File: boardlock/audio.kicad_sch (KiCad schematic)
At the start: 7 parts, among them U7 MAX98357AETE+T

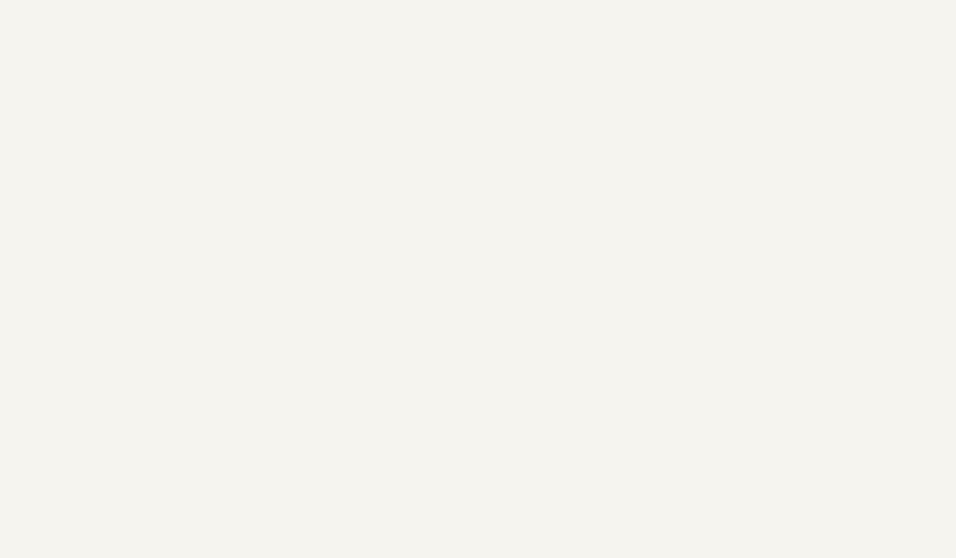
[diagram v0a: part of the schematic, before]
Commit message: modifications?
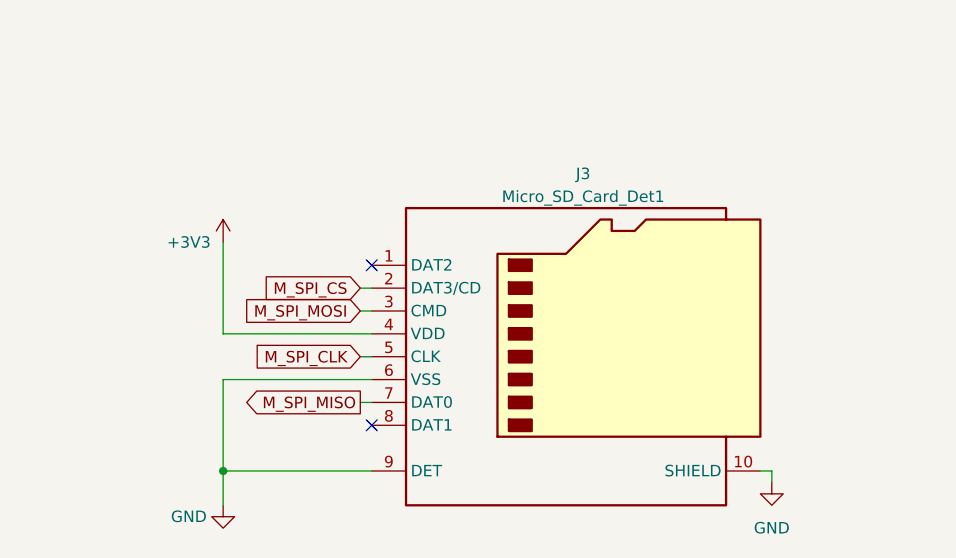
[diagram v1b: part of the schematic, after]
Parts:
- added J3: Micro_SD_Card_Det1, symbol Connector:Micro_SD_Card_Det1
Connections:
- net +3V3: now also J3.4 (VDD)
- net GND: now also J3.10 (SHIELD), J3.6 (VSS), J3.9 (DET)
- new net M_SPI_CLK: J3.5 (CLK)
- new net M_SPI_CS: J3.2 (DAT3/CD)
- new net M_SPI_MISO: J3.7 (DAT0)
- new net M_SPI_MOSI: J3.3 (CMD)
- no-connect marks 0 -> 2
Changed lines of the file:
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@@
   (junction (at 171.45 124.46) (diameter 0) (color 0 0 0 0)
   )
+  (junction (at 73.66 146.05) (diameter 0) (color 0 0 0 0)
+  )
   (junction (at 59.69 53.34) (diameter 0) (color 0 0 0 0)
   )
@@
   (junction (at 219.71 130.81) (diameter 0) (color 0 0 0 0)
   )
+  (no_connect (at 90.17 140.97))
+  (no_connect (at 90.17 123.19))
+  (wire (pts (xy 73.66 149.86) (xy 73.66 146.05))
+    (stroke (width 0) (type default))
+  )
   (wire (pts (xy 219.71 130.81) (xy 219.71 133.35))
     (stroke (width 0) (type default))
   )
+  (wire (pts (xy 134.62 146.05) (xy 134.62 147.32))
+    (stroke (width 0) (type default))
+  )
   (wire (pts (xy 41.91 39.37) (xy 52.07 39.37))
     (stroke (width 0) (type default))
@@
     (stroke (width 0) (type default))
   )
+  (wire (pts (xy 73.66 146.05) (xy 73.66 135.89))
+    (stroke (width 0) (type default))
+  )
   (wire (pts (xy 59.69 76.2) (xy 59.69 81.28))
     (stroke (width 0) (type default))
   )
+  (wire (pts (xy 88.9 125.73) (xy 90.17 125.73))
+    (stroke (width 0) (type default))
+  )
   (wire (pts (xy 59.69 76.2) (xy 62.23 76.2))
     (stroke (width 0) (type default))
@@
     (stroke (width 0) (type default))
   )
+  (wire (pts (xy 90.17 133.35) (xy 88.9 133.35))
+    (stroke (width 0) (type default))
+  )
   (wire (pts (xy 41.91 36.83) (xy 41.91 39.37))
     (stroke (width 0) (type default))
@@
     (stroke (width 0) (type default))
   )
+  (wire (pts (xy 73.66 146.05) (xy 90.17 146.05))
+    (stroke (width 0) (type default))
+  )
   (wire (pts (xy 181.61 121.92) (xy 185.42 121.92))
     (stroke (width 0) (type default))
@@
     (stroke (width 0) (type default))
   )
+  (wire (pts (xy 73.66 135.89) (xy 90.17 135.89))
+    (stroke (width 0) (type default))
+  )
+  (wire (pts (xy 90.17 128.27) (xy 88.9 128.27))
+    (stroke (width 0) (type default))
+  )
   (wire (pts (xy 97.79 77.47) (xy 101.6 77.47))
     (stroke (width 0) (type default))
@@
     (stroke (width 0) (type default))
   )
+  (wire (pts (xy 134.62 146.05) (xy 133.35 146.05))
+    (stroke (width 0) (type default))
+  )
   (wire (pts (xy 59.69 53.34) (xy 59.69 55.88))
     (stroke (width 0) (type default))
@@
     (stroke (width 0) (type default))
   )
+  (wire (pts (xy 90.17 138.43) (xy 88.9 138.43))
+    (stroke (width 0) (type default))
+  )
   (wire (pts (xy 219.71 130.81) (xy 219.71 129.54))
     (stroke (width 0) (type default))
@@
     (stroke (width 0) (type default))
   )
+  (wire (pts (xy 73.66 120.65) (xy 73.66 130.81))
+    (stroke (width 0) (type default))
+  )
   (wire (pts (xy 101.6 74.93) (xy 101.6 77.47))
     (stroke (width 0) (type default))
@@
   )
   (wire (pts (xy 97.79 60.96) (xy 104.14 60.96))
+    (stroke (width 0) (type default))
+  )
+  (wire (pts (xy 73.66 130.81) (xy 90.17 130.81))
     (stroke (width 0) (type default))
   )
@@
     (effects (font (size 1.27 1.27)) (justify left bottom))
   )
+  (global_label "M_SPI_CLK" (shape input) (at 88.9 133.35 180) (fields_autoplaced)
+    (effects (font (size 1.27 1.27)) (justify right))
+    (property "Intersheetrefs" "${INTERSHEET_REFS}" (at 75.9552 133.35 0)
+      (effects (font (size 1.27 1.27)) (justify right) hide)
+    )
+  )
+  (global_label "M_SPI_MISO" (shape output) (at 88.9 138.43 180) (fields_autoplaced)
+    (effects (font (size 1.27 1.27)) (justify right))
+    (property "Intersheetrefs" "${INTERSHEET_REFS}" (at 74.9271 138.43 0)
+      (effects (font (size 1.27 1.27)) (justify right) hide)
+    )
+  )
+  (global_label "M_SPI_CS" (shape input) (at 88.9 125.73 180) (fields_autoplaced)
+    (effects (font (size 1.27 1.27)) (justify right))
+    (property "Intersheetrefs" "${INTERSHEET_REFS}" (at 77.0438 125.73 0)
+      (effects (font (size 1.27 1.27)) (justify right) hide)
+    )
+  )
   (global_label "M_I2S_Data_Out" (shape input) (at 53.34 60.96 180) (fields_autoplaced)
     (effects (font (size 1.27 1.27)) (justify right))
@@
     )
   )
+  (global_label "M_SPI_MOSI" (shape input) (at 88.9 128.27 180) (fields_autoplaced)
+    (effects (font (size 1.27 1.27)) (justify right))
+    (property "Intersheetrefs" "${INTERSHEET_REFS}" (at 74.9271 128.27 0)
+      (effects (font (size 1.27 1.27)) (justify right) hide)
+    )
+  )
   (hierarchical_label "M_SHUTDOWN_N" (shape input) (at 177.8 134.62 180) (fields_autoplaced)
     (effects (font (size 1.27 1.27)) (justify right))
@@
     )
   )
+  (symbol (lib_id "Connector:Micro_SD_Card_Det1") (at 113.03 133.35 0) (unit 1)
+    (in_bom yes) (on_board yes) (dnp no) (fields_autoplaced)
+    (property "Reference" "J3" (at 113.665 113.03 0)
+      (effects (font (size 1.27 1.27)))
+    )
+    (property "Value" "Micro_SD_Card_Det1" (at 113.665 115.57 0)
+      (effects (font (size 1.27 1.27)))
+    )
+    (property "Footprint" "" (at 165.1 115.57 0)
+      (effects (font (size 1.27 1.27)) hide)
+    )
+    (property "Datasheet" "https://datasheet.lcsc.com/lcsc/2110151630_XKB-Connectivity-XKTF-015-N_C381082.pdf" (at 113.03 130.81 0)
+      (effects (font (size 1.27 1.27)) hide)
+    )
+    (pin "1")
+    (pin "10")
+    (pin "2")
+    (pin "3")
+    (pin "4")
+    (pin "5")
+    (pin "6")
+    (pin "7")
+    (pin "8")
+    (pin "9")
+    (instances
+      (project "boardlock"
+        (path "/e1fc29ce-837e-4062-84d8-c7e423f9eab9/1eb676fb-9e7a-4e01-ba1e-2eff94d7b66e"
+          (reference "J3") (unit 1)
+        )
+      )
+    )
+  )
+  (symbol (lib_id "power:GND") (at 73.66 149.86 0) (unit 1)
+    (in_bom yes) (on_board yes) (dnp no)
+    (property "Reference" "#PWR08" (at 73.66 156.21 0)
+      (effects (font (size 1.27 1.27)) hide)
+    )
+    (property "Value" "GND" (at 69.85 151.13 0)
+      (effects (font (size 1.27 1.27)))
+    )
+    (property "Footprint" "" (at 73.66 149.86 0)
+      (effects (font (size 1.27 1.27)) hide)
+    )
+    (property "Datasheet" "" (at 73.66 149.86 0)
+      (effects (font (size 1.27 1.27)) hide)
+    )
+    (pin "1")
+    (instances
+      (project "boardlock"
+        (path "/e1fc29ce-837e-4062-84d8-c7e423f9eab9/1eb676fb-9e7a-4e01-ba1e-2eff94d7b66e"
+          (reference "#PWR08") (unit 1)
+        )
+      )
+    )
+  )
   (symbol (lib_id "Device:C") (at 41.91 44.45 0) (unit 1)
     (in_bom yes) (on_board yes) (dnp no) (fields_autoplaced)
@@
         )
       )
+    )
+  )
+  (symbol (lib_id "power:GND") (at 134.62 147.32 0) (unit 1)
+    (in_bom yes) (on_board yes) (dnp no) (fields_autoplaced)
+    (property "Reference" "#PWR050" (at 134.62 153.67 0)
+      (effects (font (size 1.27 1.27)) hide)
+    )
+    (property "Value" "GND" (at 134.62 152.4 0)
+      (effects (font (size 1.27 1.27)))
+    )
+    (property "Footprint" "" (at 134.62 147.32 0)
+      (effects (font (size 1.27 1.27)) hide)
+    )
+    (property "Datasheet" "" (at 134.62 147.32 0)
+      (effects (font (size 1.27 1.27)) hide)
+    )
+    (pin "1")
+    (instances
+      (project "boardlock"
+        (path "/e1fc29ce-837e-4062-84d8-c7e423f9eab9/1eb676fb-9e7a-4e01-ba1e-2eff94d7b66e"
+          (reference "#PWR050") (unit 1)
+        )
+      )
+    )
+  )
+  (symbol (lib_id "power:+3V3") (at 73.66 120.65 0) (unit 1)
+    (in_bom yes) (on_board yes) (dnp no)
+    (property "Reference" "#PWR049" (at 73.66 124.46 0)
+      (effects (font (size 1.27 1.27)) hide)
+    )
+    (property "Value" "+3V3" (at 69.85 120.65 0)
+      (effects (font (size 1.27 1.27)))
+    )
+    (property "Footprint" "" (at 73.66 120.65 0)
+      (effects (font (size 1.27 1.27)) hide)
+    )
+    (property "Datasheet" "" (at 73.66 120.65 0)
+      (effects (font (size 1.27 1.27)) hide)
+    )
+    (pin "1")
+    (instances
+      (project "boardlock"
+        (path "/e1fc29ce-837e-4062-84d8-c7e423f9eab9/1eb676fb-9e7a-4e01-ba1e-2eff94d7b66e"
+          (reference "#PWR049") (unit 1)
+        )
+      )
